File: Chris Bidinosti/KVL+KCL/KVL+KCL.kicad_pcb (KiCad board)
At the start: 2 copper layers, 180 x 120 mm, 10 parts

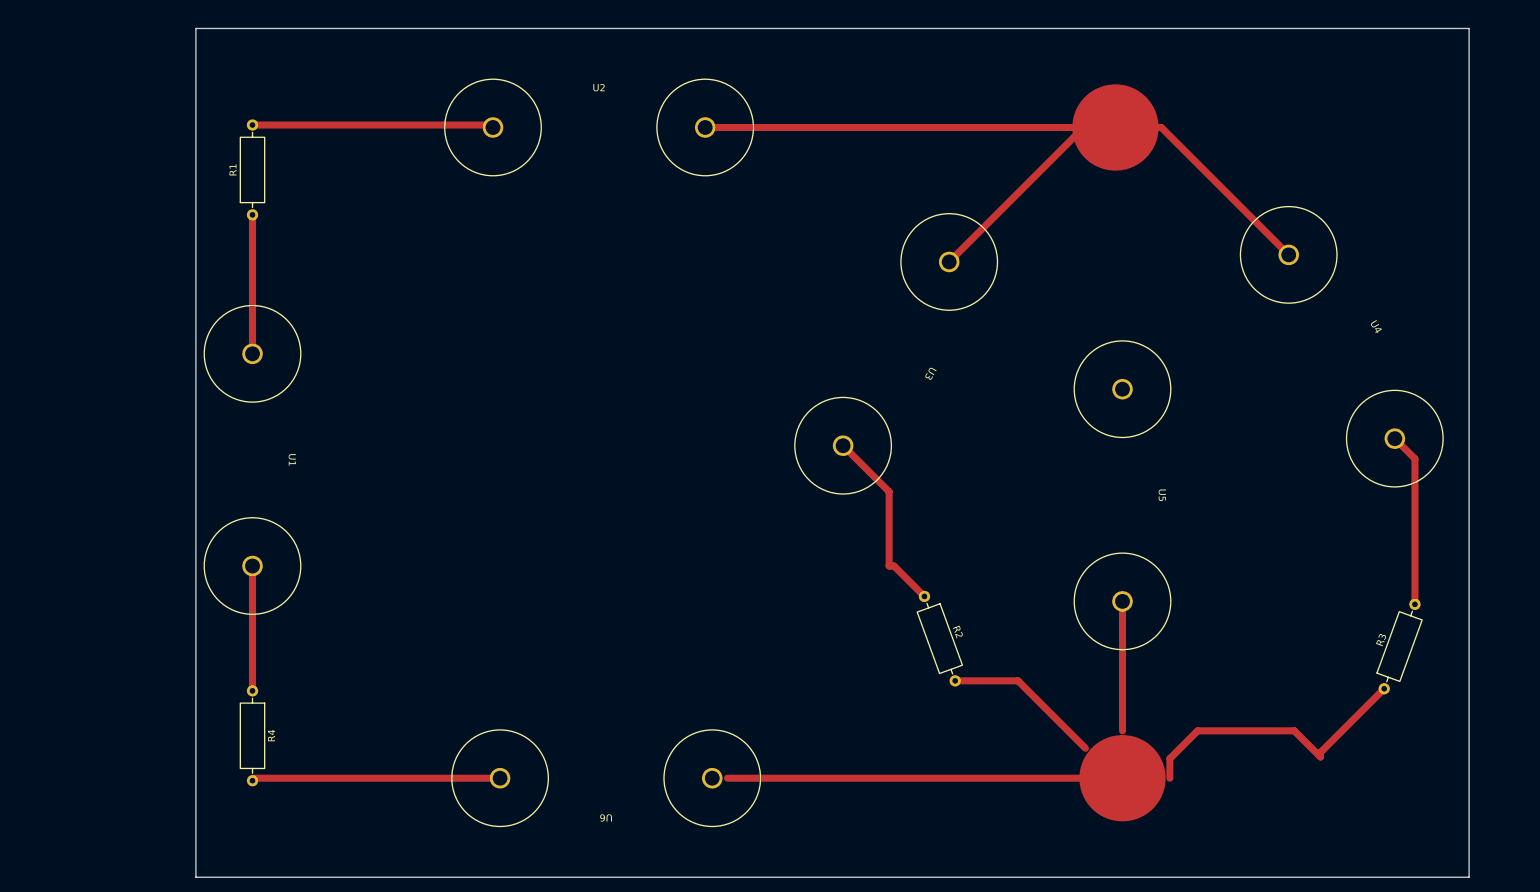
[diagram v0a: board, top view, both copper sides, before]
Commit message: Add files via upload
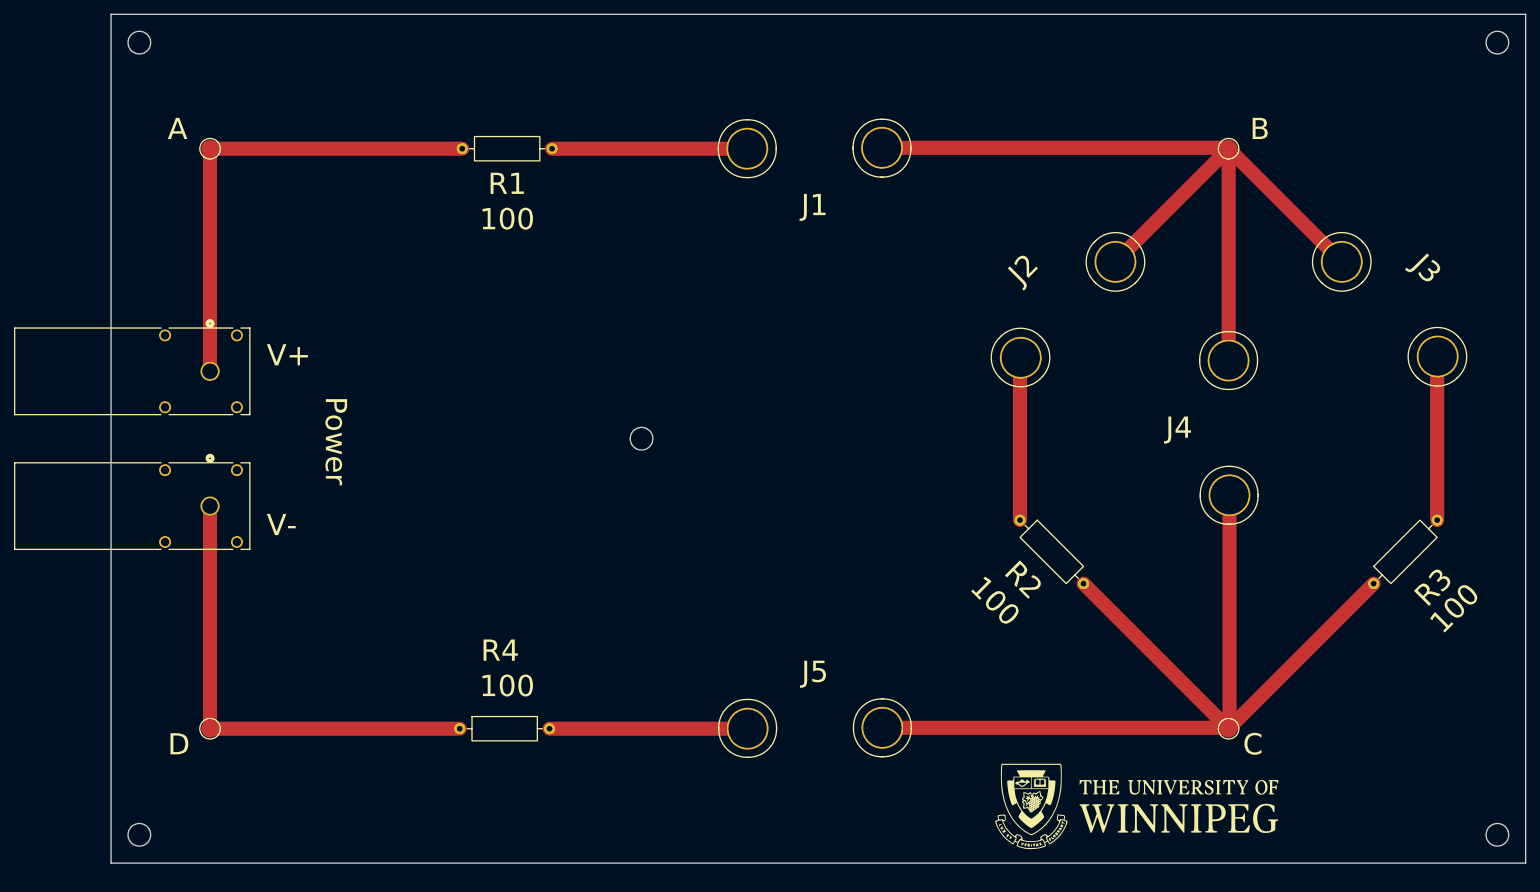
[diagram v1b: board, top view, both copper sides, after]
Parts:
- removed U2, U3, U4, U5, U6: ~, banana_connector:Red&BlackBananaConnector
- added G***: LOGO, uw_logo:uw-logo, F.Cu at (189.0, 139.0)
- added H1: MountingHole, MountingHole:MountingHole_3.2mm_M3, F.Cu at (48.0, 31.0)
- added H2: MountingHole, MountingHole:MountingHole_3.2mm_M3, F.Cu at (240.0, 31.0)
- added H3: MountingHole, MountingHole:MountingHole_3.2mm_M3, F.Cu at (240.0, 143.0)
- added H4: MountingHole, MountingHole:MountingHole_3.2mm_M3, F.Cu at (48.0, 143.0)
- added H5: MountingHole, MountingHole:MountingHole_3.2mm_M3, F.Cu at (119.0, 87.0)
- added J1: ~, jumper_connector:JumperConnector, F.Cu at (143.5, 46.0)
- added J2: ~, jumper_connector:JumperConnector, F.Cu at (179.3, 68.7)
- added J3: ~, jumper_connector:JumperConnector, F.Cu at (224.7, 68.7)
- added J4: ~, jumper_connector:JumperConnector, F.Cu at (202.0, 85.5)
- added J5: ~, jumper_connector:JumperConnector, F.Cu at (143.5, 127.9)
- added TP1: TestPoint, TestPoint:TestPoint_Pad_D2.5mm, F.Cu at (58.0, 46.0)
- added TP2: TestPoint, TestPoint:TestPoint_Pad_D2.5mm, F.Cu at (202.0, 46.0)
- added TP3: TestPoint, TestPoint:TestPoint_Pad_D2.5mm, F.Cu at (202.0, 128.0)
- added TP4: TestPoint, TestPoint:TestPoint_Pad_D2.5mm, F.Cu at (58.0, 128.0)
- U1: footprint banana_connector:Red&BlackBananaConnector -> power_connector:power_connector
- moved R1 31.1 mm to (93.7, 46.0), turned to 0 degrees
- moved R4 29.8 mm to (93.3, 128.0), turned to 0 degrees
- moved R2 17.3 mm to (172.5, 98.5), turned to -45 degrees
- moved R3 14.9 mm to (222.5, 107.5), turned to 45 degrees
- moved U1 6.71 mm to (58.0, 87.0)
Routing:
- net Net-(U2-Black): track 177.2 -> 0.00 mm
- net Net-(J1-J-): track 0.00 -> 124.3 mm
- net Net-(J4-J-): track 81.3 -> 140.0 mm
- net GND: track 17.7 -> 66.8 mm
- net +1V5: track 19.6 -> 67.1 mm
- net Net-(J5-J-): track 35.1 -> 28.0 mm
- net Net-(J1-J+): track 34.1 -> 27.6 mm
- net Net-(J2-J-): track 26.5 -> 23.0 mm
- net Net-(J3-J-): track 24.6 -> 23.2 mm
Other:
- board size 180 x 120 mm -> 200 x 120 mm
- rule pad_to_mask_clearance: 0 -> 0.1
- board text added: "${REFERENCE}"
- board text added: "A"
- board text added: "B"
- board text added: "C"
- board text added: "D"
- board text added: "Kirchoff's Loop and Junction Rule Experiment"
- board text added: "Power"
- board text added: "V 1.1, Tapendra B C, Jan 2026."
- board text added: "V+"
- board text added: "V-"
- board text added: "commissioned by C.P. Bidinosti"
